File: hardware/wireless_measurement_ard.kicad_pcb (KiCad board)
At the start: 2 copper layers, 37.1 x 21 mm, 25 parts, among them J1 Conn_01x08, J2 Tag-Connect, SW1 SW_SPDT, U1 EFM8LB1, U2 JDY-08, U3 MCP16415, U4 MAX9938, U5 MAX9938

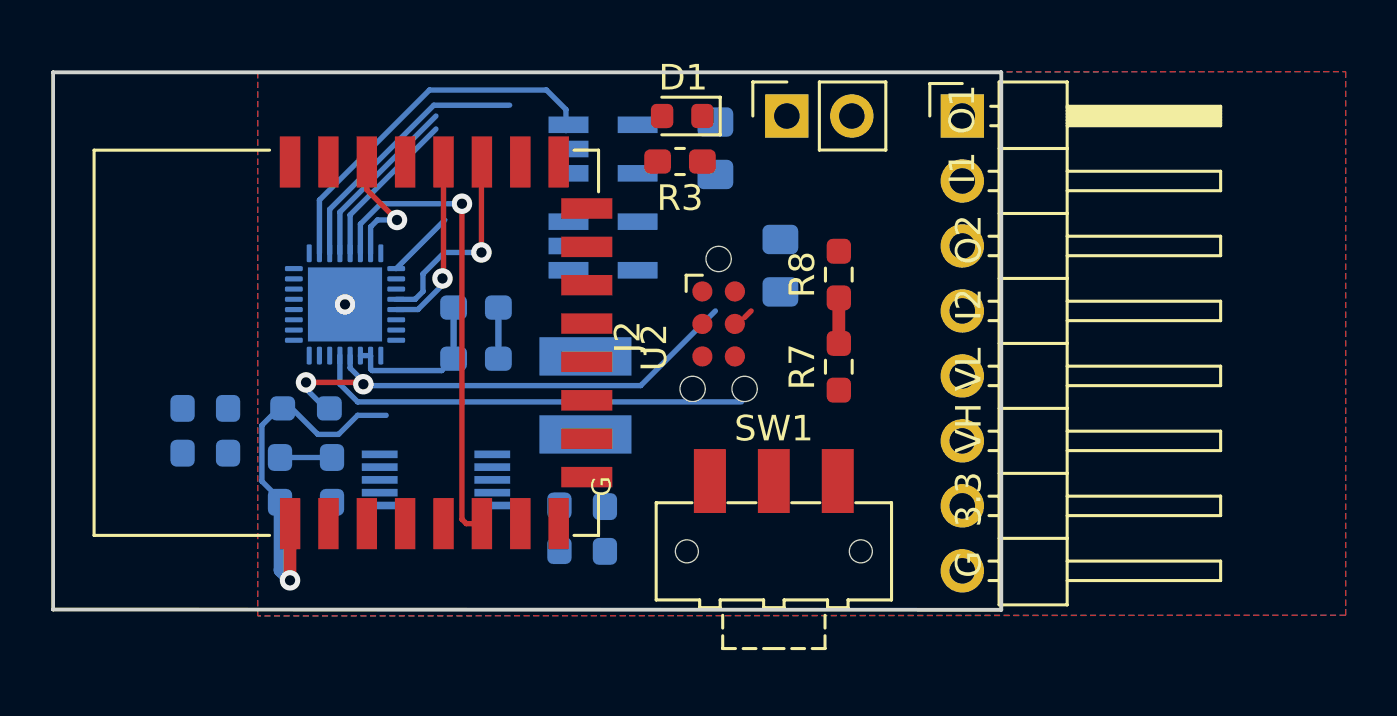
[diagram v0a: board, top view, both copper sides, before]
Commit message: completed v1
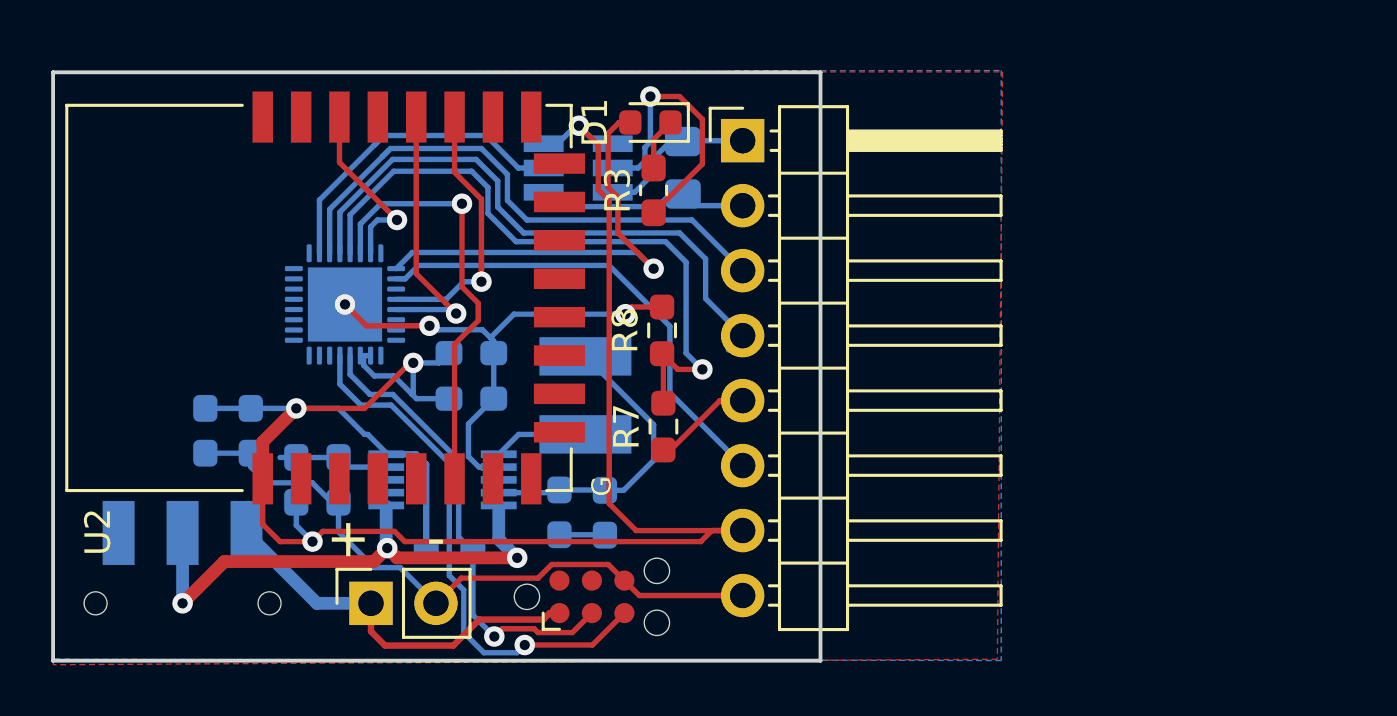
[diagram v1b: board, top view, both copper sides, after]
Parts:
- removed R2: 5R3, Resistor_SMD:R_0805_2012Metric_Pad1.15x1.40mm_HandSolder
- removed U5: MAX9938, Package_TO_SOT_SMD:SOT-23-5_HandSoldering
- R1: value 5R3 -> 1R
- SW1: moved to B.Cu
- U4: value MAX9938 -> MAX44284; footprint Package_TO_SOT_SMD:SOT-23-5_HandSoldering -> Package_TO_SOT_SMD:SOT-23-6_Handsoldering
- moved Battery1 25.0 mm to (122.4, 95.8)
- moved SW1 23.2 mm to (115.1, 95.8), turned to 180 degrees
- moved J2 11.8 mm to (131.1, 95.5), turned to 0 degrees
- moved J1 8.64 mm to (137.0, 77.7)
- moved R6 7.92 mm to (125.5, 93.7)
- moved R7 7.25 mm to (133.9, 88.8)
- moved R8 7.24 mm to (133.8, 85.1)
- moved U2 2.05 mm to (120.4, 83.8)
- moved C5 1.79 mm to (126.4, 86.0)
- moved C6 1.57 mm to (126.4, 87.8)
- moved R3 1.53 mm to (133.5, 79.6), turned to 270 degrees
- moved R1 1.48 mm to (134.6, 78.7)
- moved D1 1.27 mm to (133.3, 77.0)
- moved U4 1.22 mm to (130.5, 78.7), turned to 180 degrees
- moved C1 0.89 mm to (116.0, 89.0)
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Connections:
- J1 pad 1: C1_OUT -> C1_IN
- J1 pad 2: C1_IN -> C1_OUT
- J1 pad 3: C2_OUT -> A1
- J1 pad 4: C2_IN -> A2
- J1 pad 5: A2 -> VHIGH
- J1 pad 6: VHIGH -> A4
- R1 pad 1: C1_IN -> C1_OUT
- R1 pad 2: C1_OUT -> C1_IN
- U1 pad 26: Net-(U1-Pad26) -> A4
- U4 pad 1: GND -> +3V3
- U4 pad 3: A0 -> C1_IN
- U4 pad 5: C1_IN -> A0
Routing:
- net GND: track 2.00 -> 59.3 mm, vias 1 -> 4
- net +3V3: track 21.2 -> 77.0 mm, vias 1 -> 4
- net VIN: track 0.00 -> 33.2 mm, vias 0 -> 3
- net A4: track 0.00 -> 18.5 mm
- net A3: track 8.03 -> 25.7 mm, vias 0 -> 1
- net A2: track 6.92 -> 23.3 mm
- net BATT: track 0.00 -> 15.2 mm
- net LED: track 2.69 -> 17.7 mm, vias 0 -> 1
- net A1: track 10.4 -> 21.7 mm
- net C1_OUT: track 0.00 -> 7.89 mm
- net C1_IN: track 0.00 -> 6.34 mm
- net VHIGH: track 0.00 -> 3.96 mm
- net Net-(L1-Pad2): track 0.00 -> 3.71 mm
- net ARD_TX: track 7.03 -> 10.7 mm
- net C2D: track 17.1 -> 20.8 mm, vias 0 -> 1
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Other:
- board size 37.1 x 21 mm -> 30 x 23 mm
- board text added: "+"
- board text added: "-"
- board text added: "A1"
- board text added: "A2"
- board text added: "A4"
- board text added: "SWM-mini Sep 21"
- board text removed: "I2"
- board text removed: "O2"
- board text removed: "SWM-mini Aug 21"
- board text removed: "VL"

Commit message: mini version
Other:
- rule pad_to_mask_clearance: 0.05 -> 0
